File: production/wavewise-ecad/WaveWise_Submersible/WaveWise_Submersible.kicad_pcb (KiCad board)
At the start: 4 copper layers, 114 x 63.4 mm, 84 parts, among them J1 SMA_CONNECTOR, J10 Conn_01x03_Pin, J11 5031750600, J13 Conn_01x06_Pin, J2 SMA_CONNECTOR, J3 Conn_01x04_Pin, J4 SMA_CONNECTOR, J6 5031750200, J7 5031750800, J8 Conn_01x07_Pin, J9 5031750300, K2 AWHSH105D00G, Q2 2N2219, U1 ADS1115IDGSR, U10 AZ1117CH-3.3TRG1, U2 KP234XTMA1, U3 SI8600AC-B-ISR, U4 EZO_pH_Circuit, U5 SI8600AC-B-ISR, U6 EZO_Conductivity_Circuit, U9 Raspberry Pi Pico

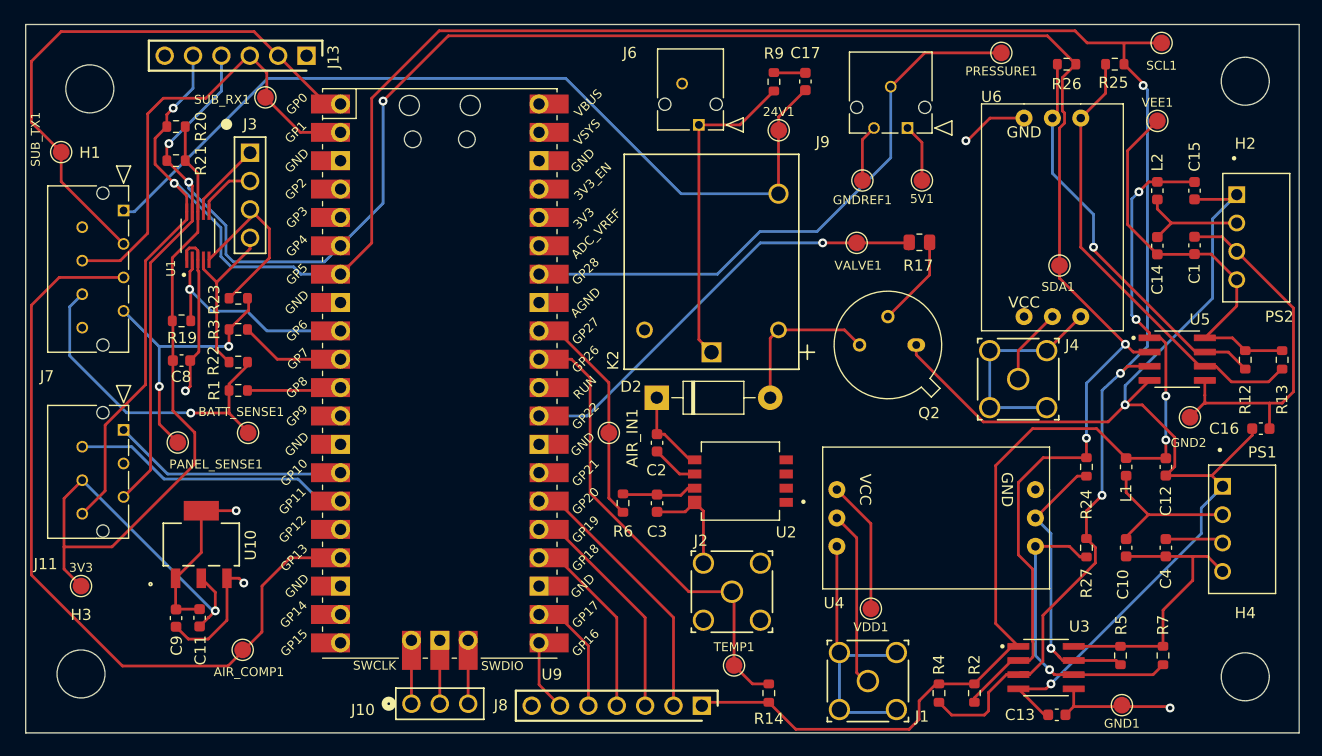
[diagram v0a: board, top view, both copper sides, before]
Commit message: Sub layout draft 2 for chiefs
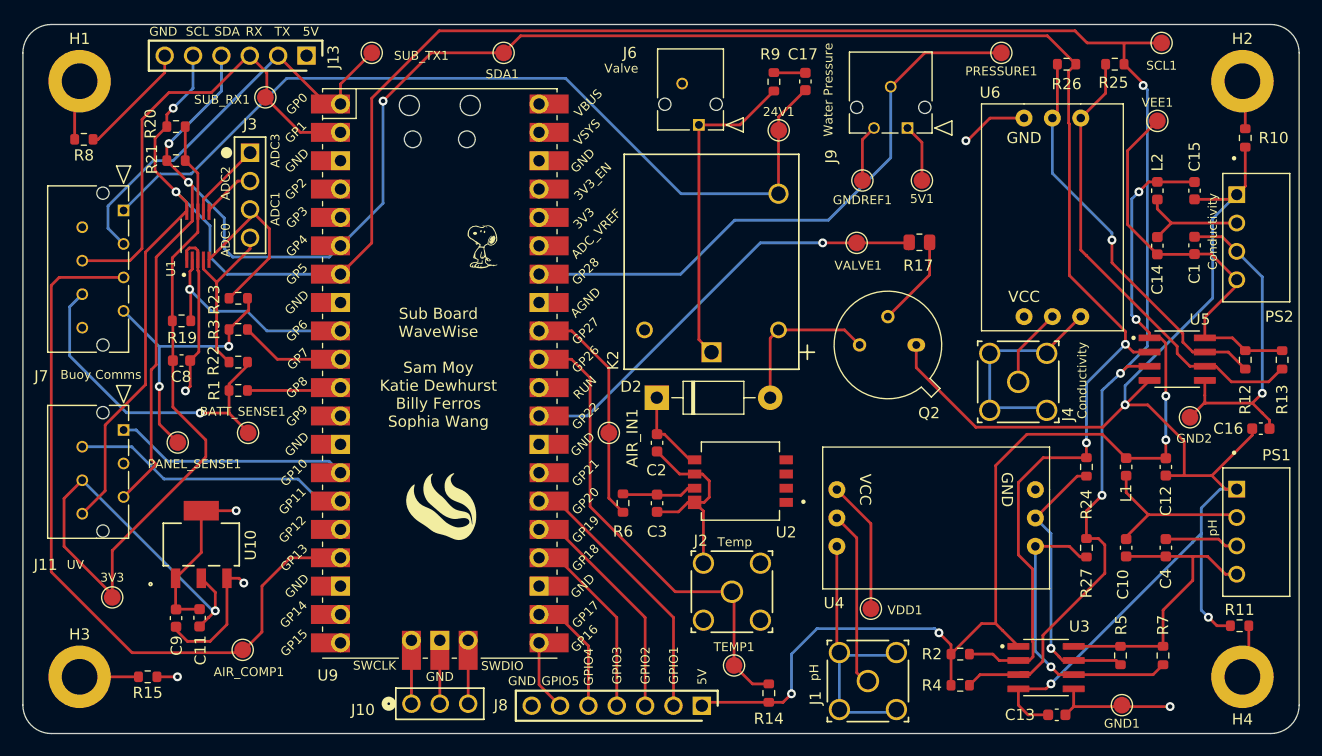
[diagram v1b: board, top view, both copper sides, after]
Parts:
- added G***: LOGO, LOGO, F.Cu at (78.5, 45.1)
- added G***: LOGO, LOGO, F.Cu at (74.6, 68.7)
- added G***: LOGO, LOGO, B.Cu at (74.4, 56.4)
- added R10: 0, Resistor_SMD:R_0603_1608Metric, F.Cu at (146.8, 35.6)
- added R11: 0, Resistor_SMD:R_0603_1608Metric, F.Cu at (146.3, 79.2)
- added R15: 0, Resistor_SMD:R_0603_1608Metric, F.Cu at (48.5, 83.8)
- added R8: 0, Resistor_SMD:R_0603_1608Metric, F.Cu at (42.8, 35.7)
- H1, H2, H3, H4: footprint MountingHole:MountingHole_4.3mm_M4 -> MountingHole:MountingHole_3.2mm_M3_DIN965_Pad
- moved SDA1 53.3 mm to (80.4, 27.9)
- moved SUB_TX1 29.2 mm to (68.6, 27.9)
- moved R2 3.72 mm to (121.3, 81.8), turned to 0 degrees
- moved 3V3 2.97 mm to (45.3, 76.7)
- moved R4 2.03 mm to (121.3, 84.6), turned to 0 degrees
- moved PS1 1.30 mm to (147.8, 70.9)
- moved H1 1.14 mm to (42.4, 30.5)
- moved H3 0.28 mm to (42.4, 83.8)
- moved H2 0.25 mm to (146.6, 30.5)
- moved H4 0.25 mm to (146.6, 83.8)
- moved J4 0.24 mm to (126.5, 57.4)
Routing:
- net GNDREF: track 154.0 -> 190.1 mm, vias 4 -> 6
- net SUB_TX: track 51.2 -> 37.9 mm
- net Net-(H1-Pad1): track 0.00 -> 6.29 mm
- net Net-(H3-Pad1): track 0.00 -> 5.27 mm
- net Net-(H4-Pad1): track 0.00 -> 4.81 mm
- net Net-(H2-Pad1): track 0.00 -> 4.36 mm
- net SCL: track 235.8 -> 231.5 mm
- net AIR_COMP: track 70.9 -> 67.3 mm
- net GND2: track 39.7 -> 36.5 mm, vias 1 -> 2
- net +5V: track 123.5 -> 126.8 mm, vias 5 -> 7
- net +3V3: track 80.2 -> 83.4 mm
- net SDA: track 216.6 -> 214.4 mm
- net VDD: track 38.3 -> 39.7 mm
- net Net-(PS1-+VIN): track 14.0 -> 15.3 mm
- net GND1: track 16.5 -> 17.9 mm
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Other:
- board size 114 x 63.4 mm -> 114.3 x 63.5 mm
- board text added: "5V"
- board text added: "ADC0"
- board text added: "ADC1"
- board text added: "ADC2"
- board text added: "ADC3"
- board text added: "Buoy Comms"
- board text added: "Conductivity"
- board text added: "GND"
- board text added: "GPIO1"
- board text added: "GPIO2"
- board text added: "GPIO3"
- board text added: "GPIO4"
- board text added: "GPIO5"
- board text added: "RX"
- board text added: "SCL"
- board text added: "SDA"
- board text added: "Sub Board WaveWise Sam Moy Katie Dewhurst Billy Ferros Sophia Wang"
- board text added: "TX"
- board text added: "Temp"
- board text added: "UV"
- board text added: "Valve"
- board text added: "Water Pressure"
- board text added: "pH"
